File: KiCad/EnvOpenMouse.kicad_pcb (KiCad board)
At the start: 2 copper layers, 34 x 106.6 mm, 117 parts, among them J1 Button, J10 0.8mm BM03B, J11 Conn_02x02_Top_Bottom, J12 0.8mm BM03B, J13 0.8mm BM03B, J2 Conn_01x03, J3 Button, J4 Conn_02x02_Top_Bottom, J5 Conn_02x02_Top_Bottom, J6 Conn_02x02_Top_Bottom, J7 Conn_02x02_Top_Bottom, J8 Conn_02x02_Top_Bottom, J9 0.8mm BM03B, SW1 SW_Push_SPDT, SW2 SW_Push_SPDT, SW3 SW_Push_SPDT, SW4 SW_Push_SPDT, SW5 SW_Push_SPDT, SW6 SW_Push_SPDT, SW7 SW_Push_SPDT, U1 AP2112K-3.3, U2 TLV70218DBVR, U3 RP2040, U4 PMW3360DM-T2QU, Y1 3225_4P 12MHz

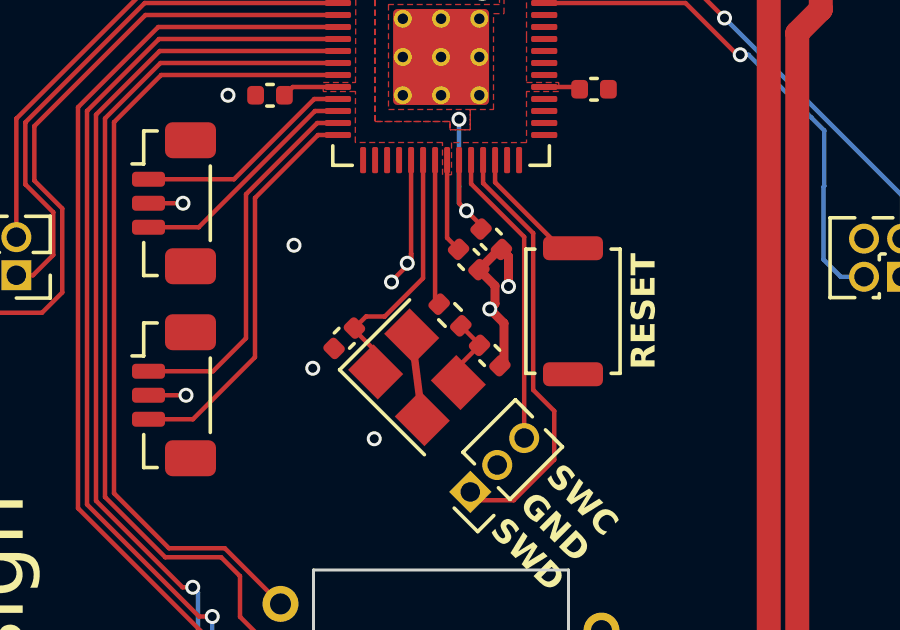
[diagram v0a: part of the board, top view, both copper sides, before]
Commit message: double checked board and tidied things up.
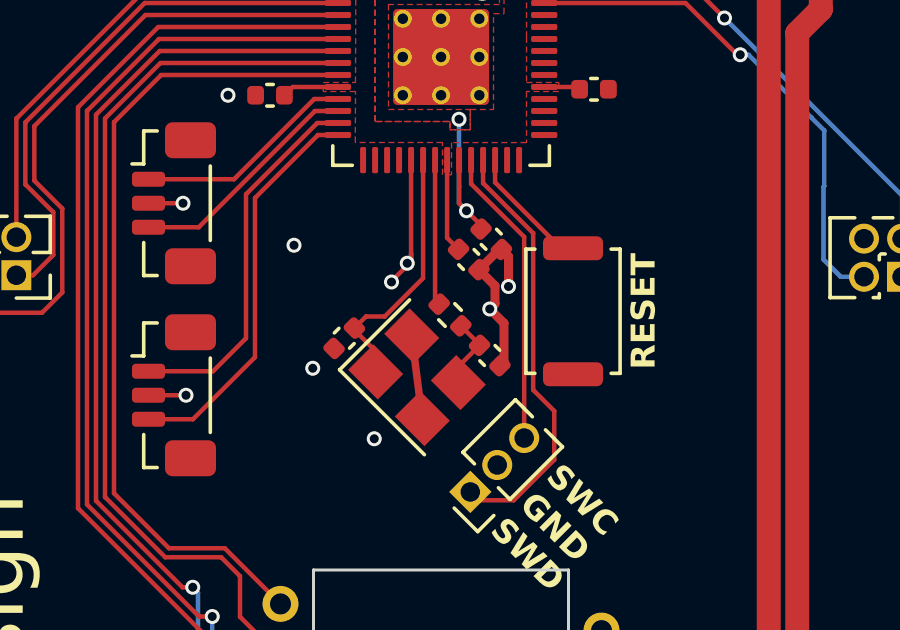
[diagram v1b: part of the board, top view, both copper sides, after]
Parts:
- R10, R9: value 27Ohms 0402 Resistor -> 27Ohms 0402 Resistor
